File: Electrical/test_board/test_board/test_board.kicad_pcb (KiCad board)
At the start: 2 copper layers, 31 parts, among them J1 Conn_01x06_Pin, J10 Conn_01x04_Socket, J11 Conn_01x06_Pin, J12 Conn_01x04_Socket, J13 Screw_Terminal_01x04, J2 Conn_01x04_Socket, J3 Conn_01x06_Pin, J4 Conn_01x04_Socket, J5 Conn_01x06_Pin, J6 Conn_01x04_Socket, J7 Conn_01x06_Pin, J8 Conn_01x04_Socket, J9 Conn_01x06_Pin

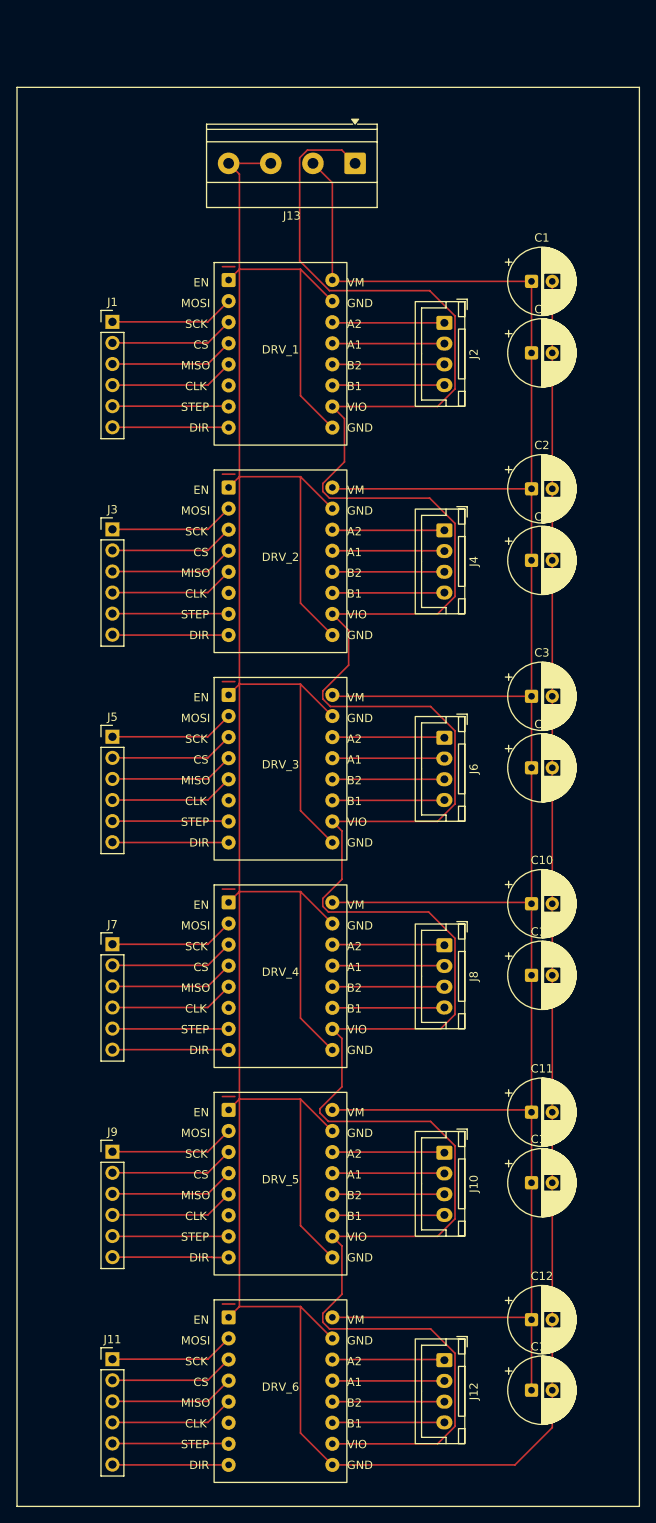
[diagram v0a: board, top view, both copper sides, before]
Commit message: Updated testboard
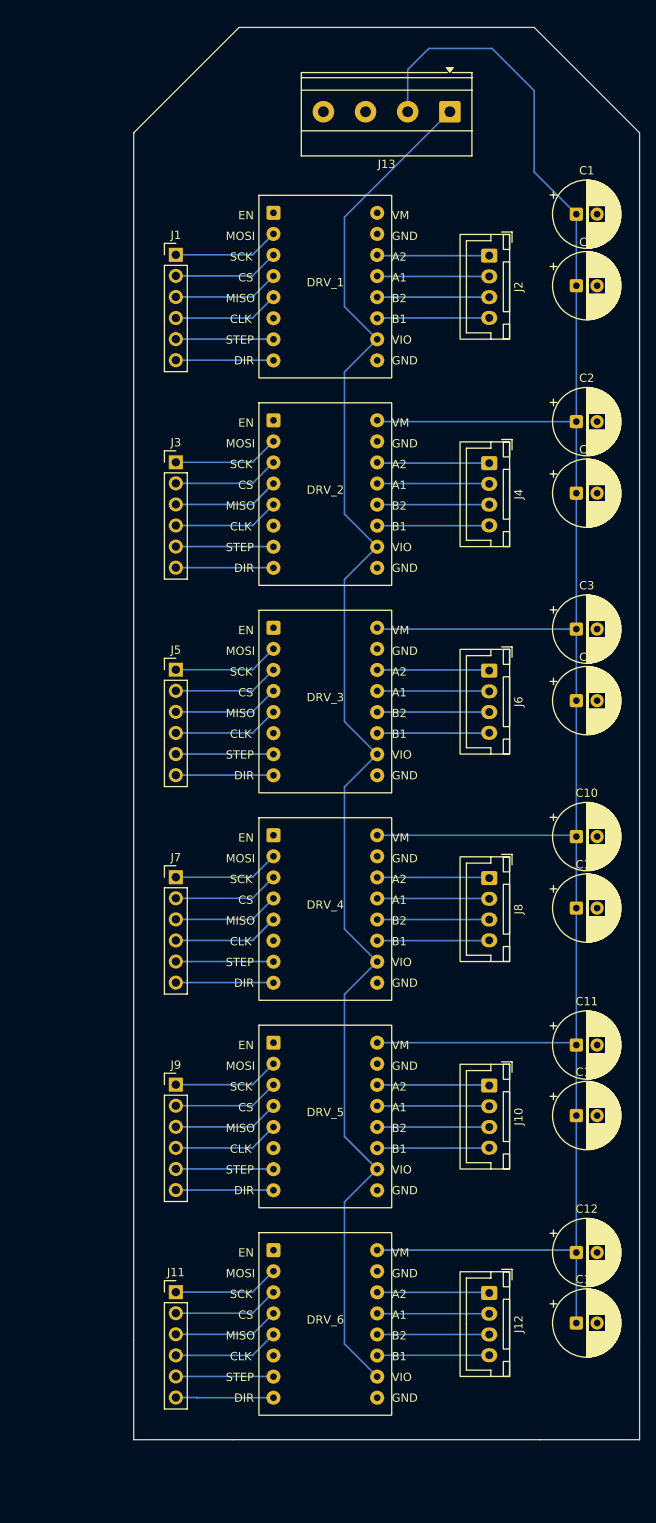
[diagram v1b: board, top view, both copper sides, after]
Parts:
- moved J13 13.0 mm to (137.2, 27.9)
- moved J1 11.1 mm to (104.1, 45.2)
- moved J3 11.1 mm to (104.1, 70.2)
- moved J5 11.1 mm to (104.1, 95.2)
- moved J11 11.1 mm to (104.1, 170.2)
- moved J7 11.1 mm to (104.1, 120.2)
- moved J9 11.1 mm to (104.1, 145.2)
- moved DRV_4 9.73 mm to (122.2, 124.0)
- moved C1 9.73 mm to (152.4, 40.3)
- moved C11 9.73 mm to (152.4, 140.4)
- moved C12 9.73 mm to (152.4, 165.4)
- moved C13 9.73 mm to (152.4, 123.9)
- moved C14 9.73 mm to (152.4, 148.9)
- moved C15 9.73 mm to (152.4, 173.9)
- moved C5 9.73 mm to (152.4, 73.9)
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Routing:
- net GND: track 521.8 -> 0.00 mm
- net +3.3V: track 335.9 -> 175.6 mm
- net Net-(DRV_5-Pin_15): track 14.0 -> 11.8 mm
- net Net-(DRV_6-Pin_7): track 15.0 -> 12.8 mm
- net Net-(DRV_6-Pin_5): track 15.0 -> 12.8 mm
- net Net-(DRV_5-Pin_7): track 15.0 -> 12.8 mm
- net Net-(DRV_5-Pin_5): track 15.0 -> 12.8 mm
- net Net-(DRV_4-Pin_9): track 15.0 -> 12.8 mm
- net Net-(DRV_4-Pin_5): track 15.0 -> 12.8 mm
- net Net-(DRV_3-Pin_9): track 15.0 -> 12.8 mm
- net Net-(DRV_3-Pin_5): track 15.0 -> 12.8 mm
- net Net-(DRV_2-Pin_9): track 15.0 -> 12.8 mm
- net Net-(DRV_2-Pin_5): track 15.0 -> 12.8 mm
- net Net-(DRV_1-Pin_9): track 15.0 -> 12.8 mm
- net Net-(DRV_1-Pin_7): track 15.0 -> 12.8 mm
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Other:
- board outline added: 61 x 170.2 mm

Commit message: Finished testboard
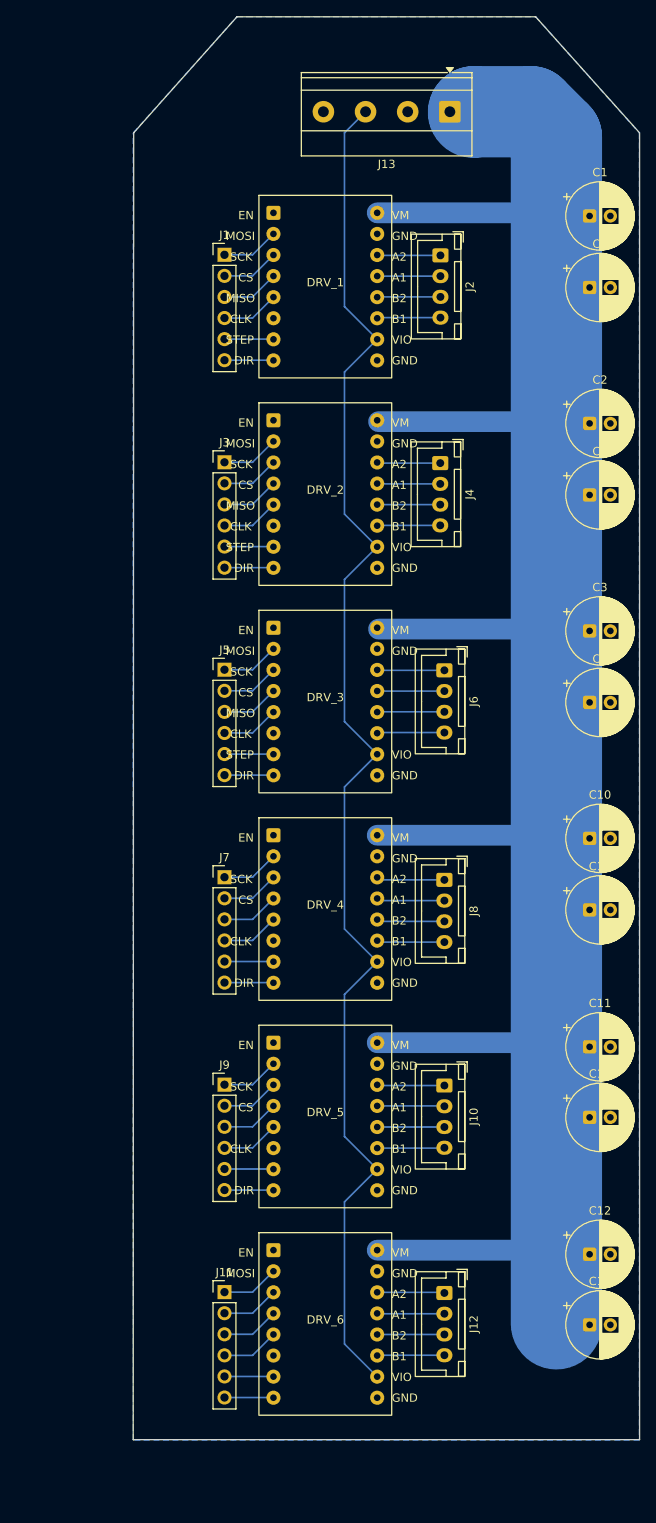
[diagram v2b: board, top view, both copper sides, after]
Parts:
- moved J4 5.90 mm to (136.0, 70.3)
- moved J2 5.88 mm to (136.0, 45.2)
- moved J1 5.86 mm to (110.0, 45.2)
- moved J11 5.86 mm to (110.0, 170.2)
- moved J3 5.86 mm to (110.0, 70.2)
- moved J5 5.86 mm to (110.0, 95.2)
- moved J7 5.86 mm to (110.0, 120.2)
- moved J9 5.86 mm to (110.0, 145.2)
- moved J8 5.41 mm to (136.5, 120.5)
- moved J6 5.40 mm to (136.5, 95.2)
- moved J10 5.40 mm to (136.5, 145.3)
- moved J12 5.40 mm to (136.5, 170.3)
- moved C11 1.61 mm to (154.0, 140.6)
- moved C12 1.61 mm to (154.0, 165.6)
- moved C13 1.61 mm to (154.0, 124.1)
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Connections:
- J13 pad 1: +3.3V -> +24V
- J13 pad 2: +24V -> GND
- J13 pad 3: GND -> +3.3V
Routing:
- net +24V: track 294.7 -> 319.3 mm
- net Net-(DRV_2-Pin_6): track 13.5 -> 7.63 mm
- net Net-(DRV_2-Pin_10): track 13.5 -> 7.60 mm
- net Net-(DRV_2-Pin_12): track 13.5 -> 7.62 mm
- net Net-(DRV_2-Pin_8): track 13.5 -> 7.62 mm
- net Net-(DRV_1-Pin_6): track 13.5 -> 7.67 mm
- net Net-(DRV_1-Pin_12): track 13.5 -> 7.65 mm
- net Net-(DRV_1-Pin_10): track 13.5 -> 7.64 mm
- net Net-(DRV_1-Pin_8): track 13.5 -> 7.65 mm
- net Net-(DRV_6-Pin_13): track 11.8 -> 5.97 mm
- net Net-(DRV_4-Pin_15): track 11.8 -> 5.97 mm
- net Net-(DRV_1-Pin_9): track 12.8 -> 6.94 mm
- net Net-(DRV_1-Pin_7): track 12.8 -> 6.94 mm
- net Net-(DRV_1-Pin_5): track 12.8 -> 6.94 mm
- net Net-(DRV_1-Pin_3): track 12.8 -> 6.94 mm
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- added copper zone on B.Cu, net GND
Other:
- board size 61 x 170.2 mm -> 61 x 171.5 mm
